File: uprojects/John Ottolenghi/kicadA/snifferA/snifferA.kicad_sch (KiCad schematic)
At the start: 64 parts, among them J1 DHT22, J10 ZP07, J11 DCJ200-10-A-XX-K_REVA, J2 Conn_01x10, J3 CCS811_CJMCU, J4 Conn_01x08, J5 Conn_01x08, J6 Conn_02x18_Odd_Even, J7 Conn_01x08, J8 Conn_01x08, J9 Conn_01x08, U1 MQ-131-H, U10 MQ-131-L, U11 ZE-03, U12 ZE08-CH20, U13 ZP07, U14 SM4-NO2-20, U15 MQ-07, U16 YAAJ_DCDC_StepDown_LM2596, U2 MQ-135, U3 MQ-136, U4 MQ-137, U5 MQ-02, U6 MQ-04, U7 MQ-06, U8 MQ-08, U9 YAAJ_DCDC_StepDown_LM2596

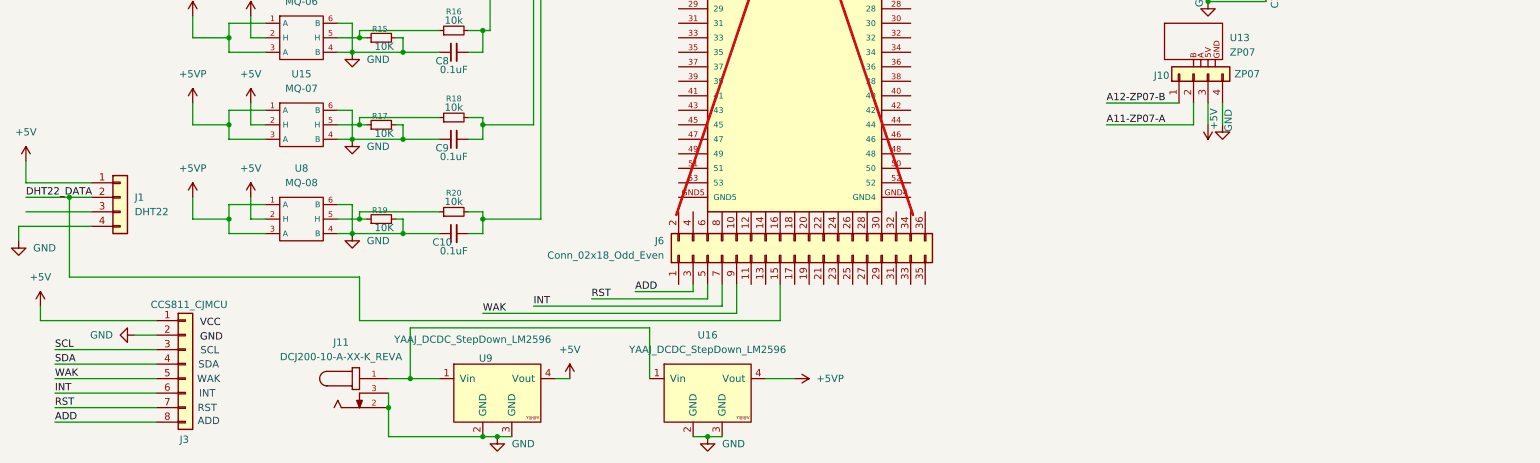
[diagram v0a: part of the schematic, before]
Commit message: Update 9 mar 2026
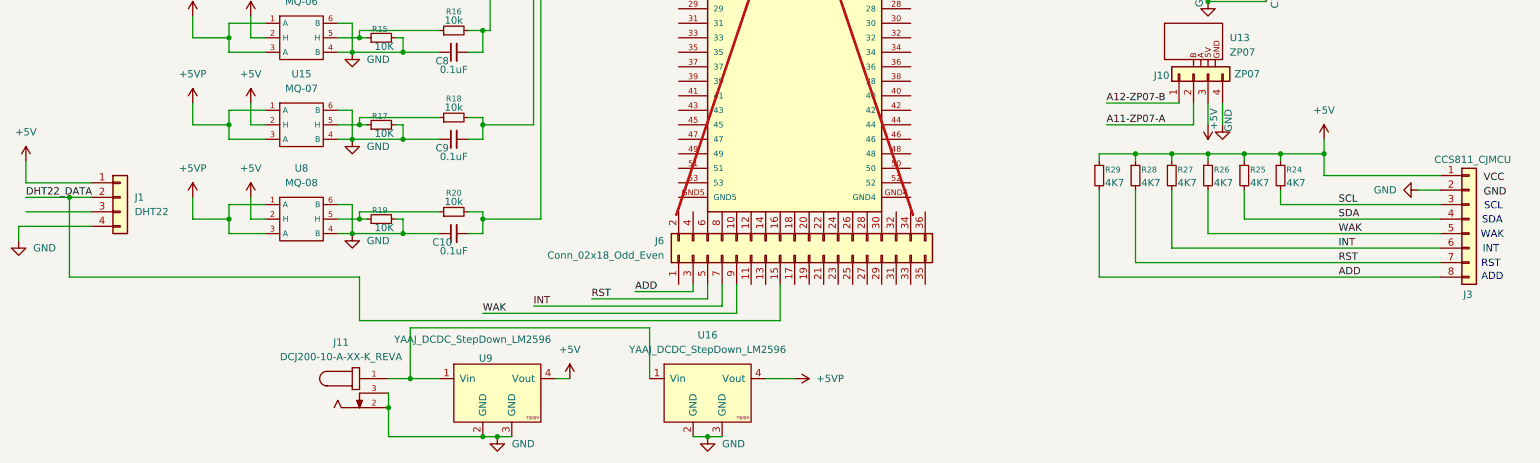
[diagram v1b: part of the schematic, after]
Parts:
- added R24, R25, R26, R27, R28, R29: 4K7, Resistor_SMD:R_0603_1608Metric, symbol Device:R_Small
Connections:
- net +5V: now also R24.1, R25.1, R26.1, R27.1, R28.1, R29.1
- net ADD: now also R29.2
- net INT: now also R27.2
- net RST: now also R28.2
- net SCL: now also R24.2
- net SDA: now also R25.2
- net WAK: now also R26.2
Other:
- moved on the sheet: J3
